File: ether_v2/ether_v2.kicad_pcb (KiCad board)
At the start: 2 copper layers, 50.3 x 110 mm, 82 parts, among them J1 PJ398SM, J10 PJ398SM, J11 PJ398SM, J12 PJ398SM, J13 PJ398SM, J14 PJ398SM, J15 PJ398SM, J16 PJ398SM, J17 SS65100-024F, J18 SS65100-024F, J19 Power, J2 PJ398SM, J20 Conn_01x03, J3 PJ398SM, J4 PJ398SM, J5 PJ398SM, J6 PJ398SM, J7 PJ398SM, J8 PJ398SM, J9 PJ398SM, U1 TL074, U2 TL074, U3 TL074, U4 TL074

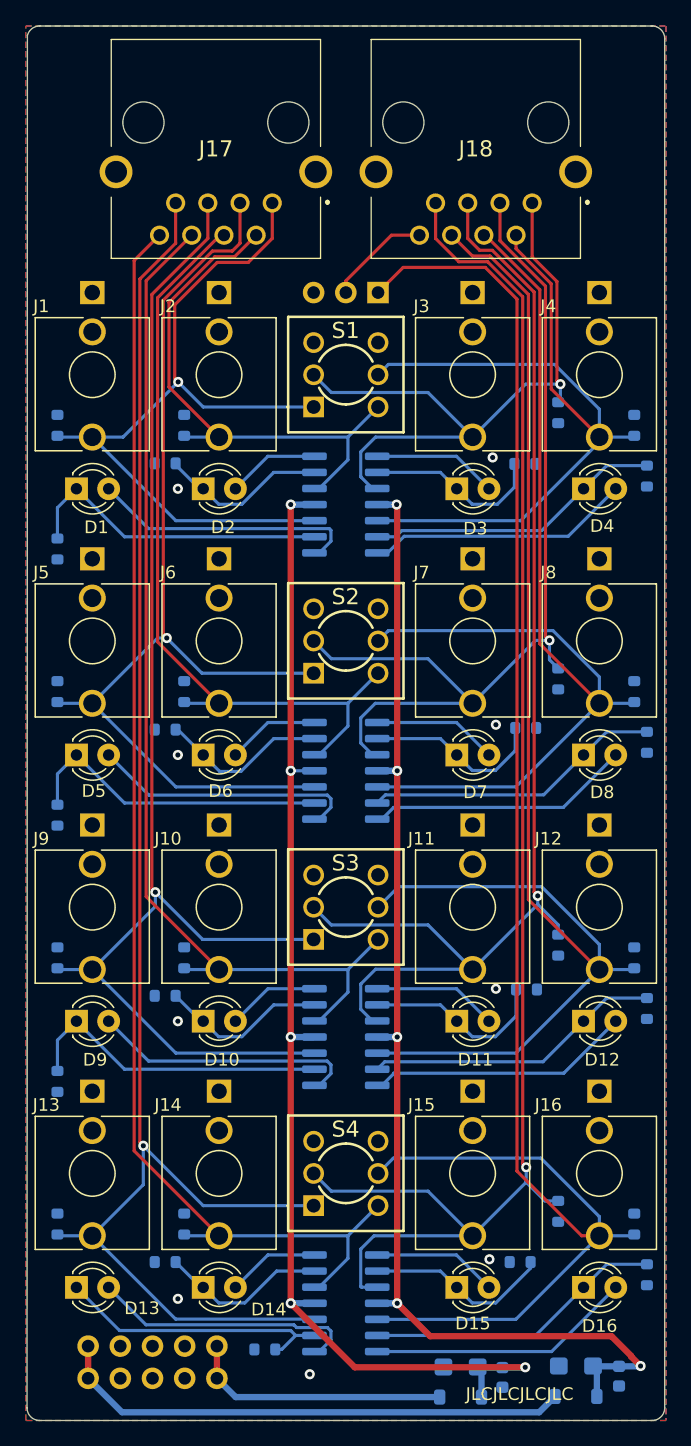
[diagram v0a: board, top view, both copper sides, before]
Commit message: fix bad merge
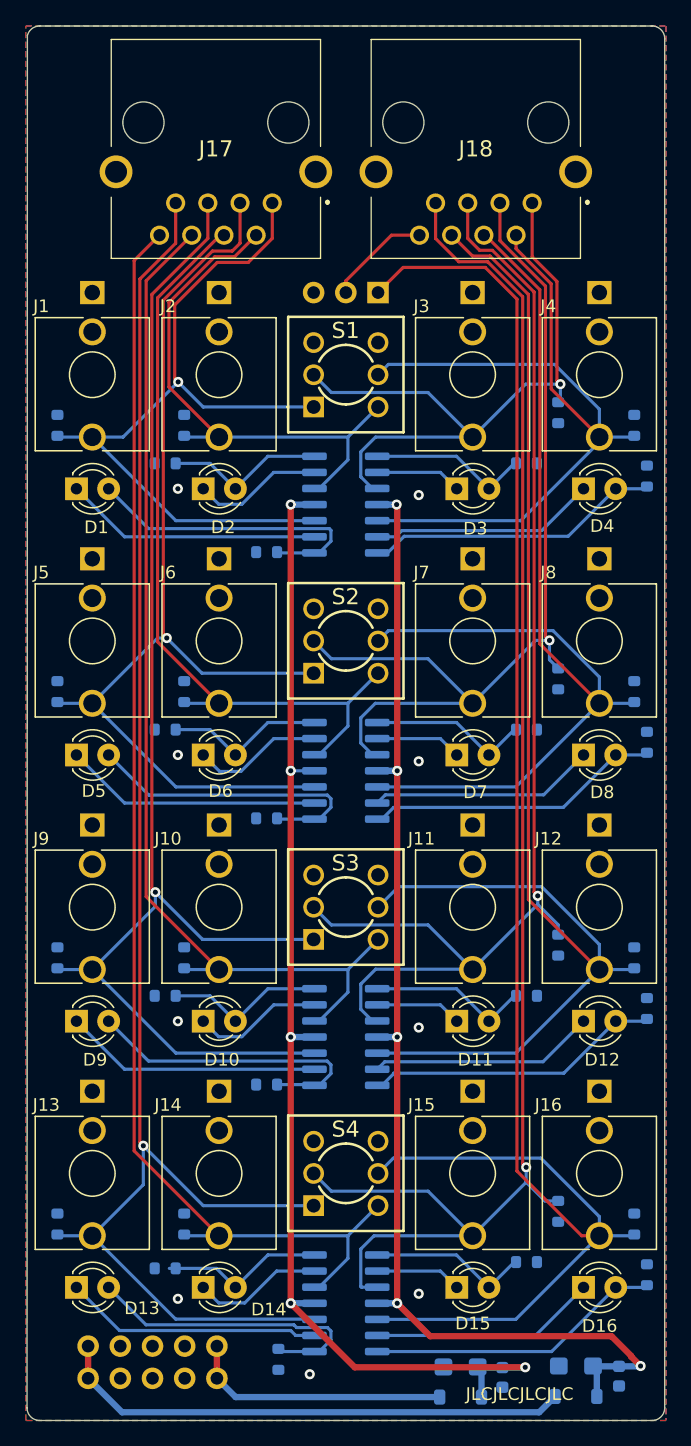
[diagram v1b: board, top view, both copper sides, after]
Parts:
- moved R13 16.5 mm to (49.0, 92.5), turned to 0 degrees
- moved R25 16.5 mm to (49.0, 113.5), turned to 0 degrees
- moved R9 16.5 mm to (49.0, 71.5), turned to 0 degrees
- moved R29 1.33 mm to (49.9, 135.2), turned to 90 degrees
- moved R26 0.50 mm to (69.5, 106.5), turned to 0 degrees
- moved R30 0.50 mm to (69.5, 127.5)
- moved R31 0.50 mm to (41.0, 128.0), turned to 0 degrees
- moved R14 0.15 mm to (69.5, 85.5), turned to 0 degrees
- moved R10 0.13 mm to (69.5, 64.5), turned to 0 degrees
- turned R11 to 0 degrees
- turned R15 to 0 degrees
- turned R27 to 0 degrees
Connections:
- R10 pad 1: GND -> Net-(D3-A)
- R10 pad 2: Net-(D3-K) -> GND
- R11 pad 1: Net-(D2-K) -> GND
- R11 pad 2: GND -> Net-(D2-A)
- R12 pad 1: GND -> Net-(D4-A)
- R12 pad 2: Net-(D4-K) -> GND
- R13 pad 1: Net-(D5-K) -> GND
- R13 pad 2: GND -> Net-(D5-A)
- R14 pad 1: GND -> Net-(D7-A)
- R14 pad 2: Net-(D7-K) -> GND
- R15 pad 1: Net-(D6-K) -> GND
- R15 pad 2: GND -> Net-(D6-A)
- R16 pad 1: GND -> Net-(D8-A)
- R16 pad 2: Net-(D8-K) -> GND
- R25 pad 1: Net-(D9-K) -> GND
- R25 pad 2: GND -> Net-(D9-A)
- R26 pad 1: GND -> Net-(D11-A)
- R26 pad 2: Net-(D11-K) -> GND
- R27 pad 1: Net-(D10-K) -> GND
- R27 pad 2: GND -> Net-(D10-A)
- R28 pad 1: GND -> Net-(D12-A)
- R28 pad 2: Net-(D12-K) -> GND
- R29 pad 1: Net-(D13-K) -> GND
- R29 pad 2: GND -> Net-(D13-A)
- R30 pad 1: GND -> Net-(D15-A)
- R30 pad 2: Net-(D15-K) -> GND
- R31 pad 1: Net-(D14-K) -> GND
- R31 pad 2: GND -> Net-(D14-A)
- R32 pad 1: GND -> Net-(D16-A)
- R32 pad 2: Net-(D16-K) -> GND
- R9 pad 2: Net-(D1-K) -> Net-(D1-A)
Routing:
- net Net-(D11-K): track 14.8 -> 6.81 mm
- net Net-(D15-K): track 14.8 -> 6.81 mm
- net Net-(D7-K): track 14.4 -> 6.81 mm
- net Net-(D3-K): track 14.3 -> 6.81 mm
- net Net-(D14-A): track 7.30 -> 13.1 mm
- net Net-(D8-K): track 23.6 -> 17.8 mm
- net Net-(D4-K): track 23.6 -> 17.8 mm
- net Net-(D16-K): track 23.6 -> 17.8 mm
- net Net-(D12-K): track 23.6 -> 17.8 mm
- net Net-(D6-A): track 7.30 -> 12.8 mm
- net Net-(D2-A): track 7.30 -> 12.8 mm
- net Net-(D10-A): track 7.30 -> 12.8 mm
- net Net-(D9-K): track 24.9 -> 20.3 mm
- net Net-(D5-K): track 24.9 -> 20.3 mm
- net Net-(D1-K): track 24.9 -> 20.3 mm
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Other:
- board text added: "Ether Twin v2.2 2024-03-01"
- board text removed: "Ether Twin v2.3 2024-03-17"
